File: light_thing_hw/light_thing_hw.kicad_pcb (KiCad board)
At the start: 2 copper layers, 50 x 50 mm, 58 parts, among them J1 CONNECTORS, J2 Li-Ion Battery, J3 ADDR_LED_PANEL_1_CONNECTORS, J4 ADDR_LED_PANEL_2_CONNECTORS, J5 MIC_CONN, Q1 MMBF170, Q2 BSS83P, SW1 ST_USER_BUTTON1, SW2 ST_RESET_BUTTON, U1 BC832-V1, U2 LSM6DS3, U3 MCP73833T-FCI_UN, U4 LMR62421XMF, U5 LP38511MRX-ADJ_NOPB, U5A1 STM32L452RETx

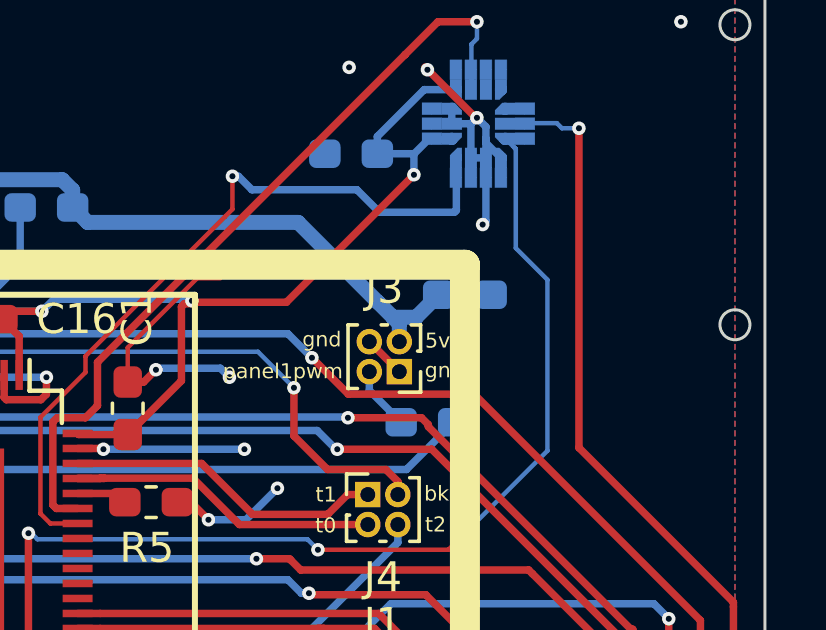
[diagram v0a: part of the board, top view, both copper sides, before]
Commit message: hw updates. sent to print
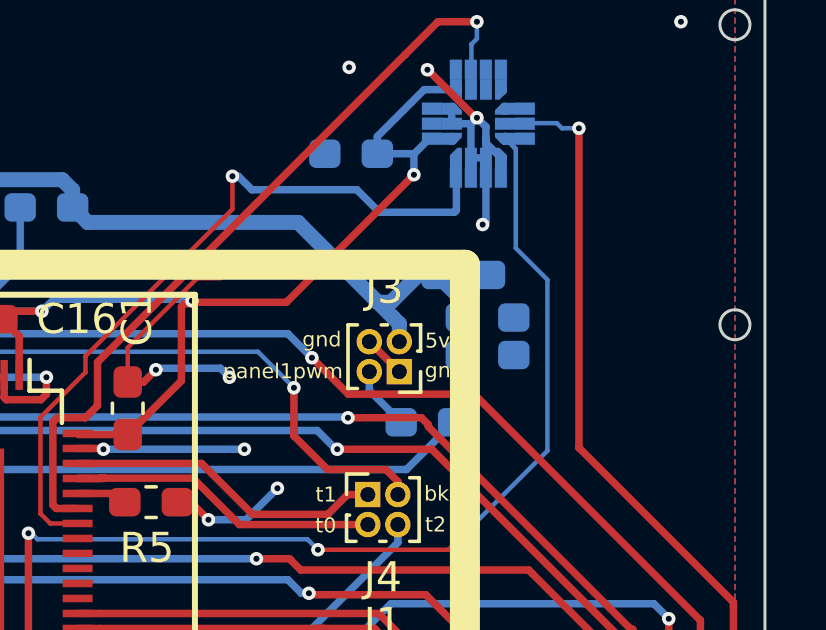
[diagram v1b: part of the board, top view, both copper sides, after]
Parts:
- added C19: 220uF, Capacitor_SMD:C_0603_1608Metric_Pad1.05x0.95mm_HandSolder, B.Cu at (160.3, 78.3)
- added C20: 220uF, Capacitor_SMD:C_0603_1608Metric_Pad1.05x0.95mm_HandSolder, B.Cu at (160.3, 77.0)
- C7: value 1000uF -> 220uF
- moved C7 0.66 mm to (159.4, 75.6)
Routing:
- net +5V: track 24.8 -> 28.3 mm
